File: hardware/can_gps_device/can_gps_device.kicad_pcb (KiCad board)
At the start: 2 copper layers, 70 x 55 mm, 79 parts, among them J1 AMP_Superseal_9-6437287-8, J2 TC2030, U1 STM32F042K6Ux, U2 TLE42744DV33ATMA1, U3 TCAN3403DRQ1, U4 R-78E5.0-0.5, Y1 ECS-160-10-36Q-AES-TR

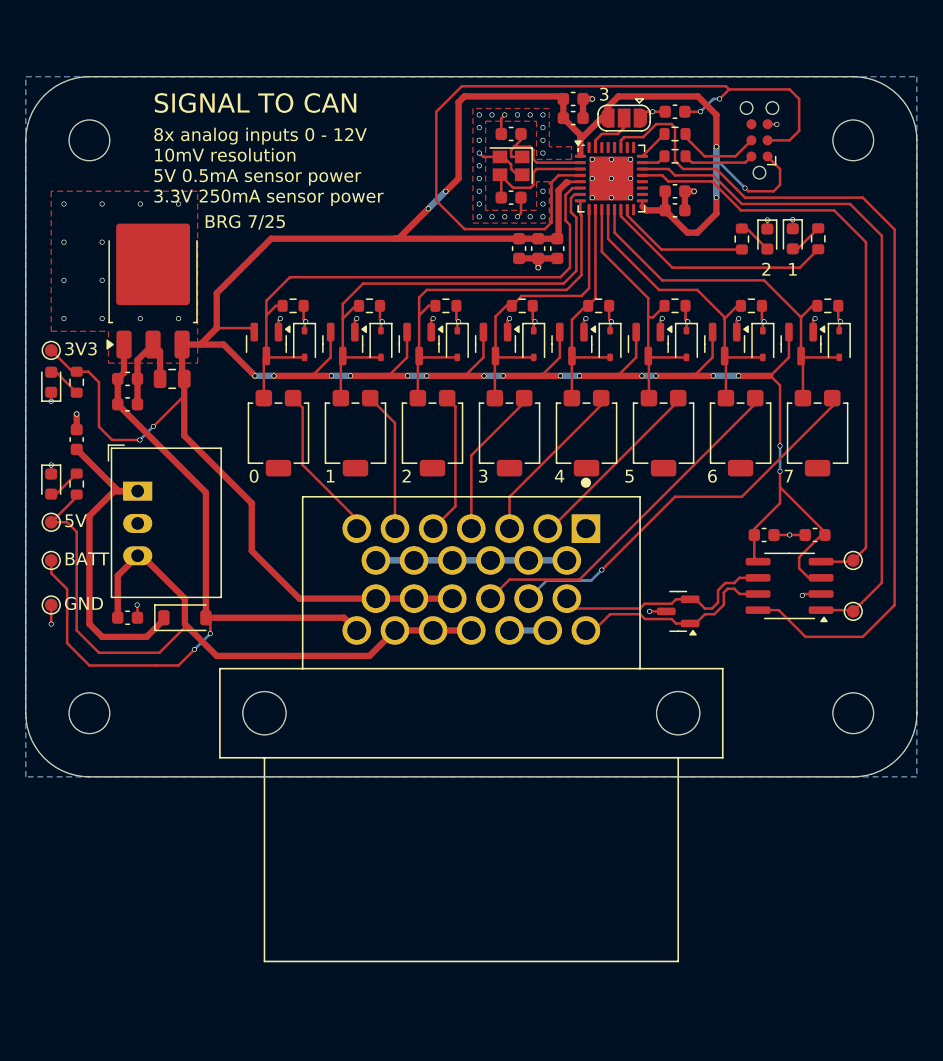
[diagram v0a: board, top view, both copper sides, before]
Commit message: Schematic Initial Rev
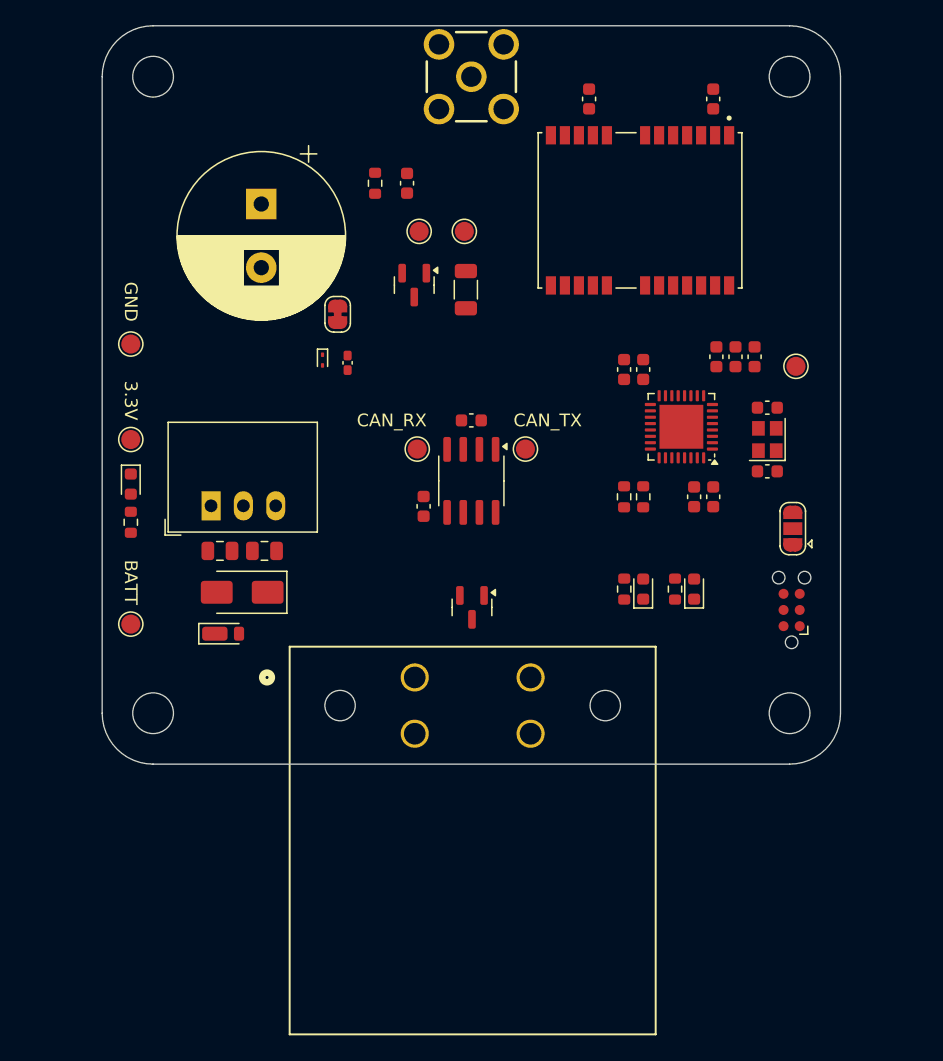
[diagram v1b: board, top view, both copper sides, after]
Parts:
- removed D10, D11, D12, D17, D18, D19, D20, D9: BAT54S, Package_TO_SOT_SMD:SOT-23
- removed D13, D14, D15, D16: PESD3V3L1BA, Diode_SMD:D_SOD-323
- removed D21: CDBW140-G, Diode_SMD:D_SOD-123
- removed D22: LED, LED_SMD:LED_0603_1608Metric
- removed R10, R11, R12, R13, R8, R9: 6.8k, Resistor_SMD:R_0603_1608Metric
- removed R14: 1k, Resistor_SMD:R_0603_1608Metric
- removed RV1, RV2, RV3, RV4, RV5, RV6, RV7, RV8: 3314G-1-503E, Potentiometer_SMD:Potentiometer_Bourns_3314G_Vertical
- removed TP3: 3.3V, TestPoint:TestPoint_Pad_D1.0mm
- removed TP4: CAN_TX, TestPoint:TestPoint_Pad_D1.0mm
- removed TP5: CAN_RX, TestPoint:TestPoint_Pad_D1.0mm
- removed TP6: TestPoint, TestPoint:TestPoint_Pad_D1.0mm
- added 3.3V1: TestPoint, TestPoint:TestPoint_Pad_D1.5mm, F.Cu at (123.2, 103.5)
- added BATT1: TestPoint, TestPoint:TestPoint_Pad_D1.5mm, F.Cu at (123.2, 118.0)
- added GND1: TestPoint, TestPoint:TestPoint_Pad_D1.5mm, F.Cu at (123.2, 96.0)
- added J3: SMA-J-P-X-RA-TH1, can_gps_device:SAMTEC_SMA-J-P-X-RA-TH1, F.Cu at (150.0, 75.0)
- added JP2: Jumper_2_Bridged, Jumper:SolderJumper-2_P1.3mm_Bridged_RoundedPad1.0x1.5mm, F.Cu at (139.5, 93.7)
- added L1: LQG15HN27NJ02D, Inductor_SMD:L_0402_1005Metric_Pad0.77x0.64mm_HandSolder, F.Cu at (140.3, 97.5)
- added MCU_RX1: TestPoint, TestPoint:TestPoint_Pad_D1.5mm, F.Cu at (149.4, 87.2)
- added MCU_TX1: TestPoint, TestPoint:TestPoint_Pad_D1.5mm, F.Cu at (145.9, 87.2)
- added RESET1: TestPoint, TestPoint:TestPoint_Pad_D1.5mm, F.Cu at (175.5, 97.8)
- C10, C11: value 1uF -> 0.1uF
- C12: value 0.1uF -> 1uF
- C13: value 22uF -> 0.1uF; footprint Capacitor_SMD:C_0805_2012Metric -> Capacitor_SMD:C_0603_1608Metric
- C14: value 0.1uF -> 100nF 16V X7R
- C15: value 0.1uF -> FYD0H104ZF; footprint Capacitor_SMD:C_0603_1608Metric -> Capacitor_THT:CP_Radial_D13.0mm_P5.00mm
- C16, C17: footprint Capacitor_SMD:C_0603_1608Metric -> Capacitor_SMD:C_0805_2012Metric
- C2: value 4.7uF -> 0.1uF
- C4: value 0.1uF -> 4.7uF
- C6: value 0.1uF -> 12pF
- C7: value 12pF -> 10nF
- C8: value 10nF -> 12pF
- C9: value 12pF -> 1uF
- D1, D2: value LED -> Green LED
- D3: value LED -> NUP2105L; footprint LED_SMD:LED_0603_1608Metric -> Package_TO_SOT_SMD:SOT-23
- D4: value NUP2105L -> BAT54A
- D5: value PESD3V3L1BA -> ESD9R3.3ST5G; footprint Diode_SMD:D_SOD-323 -> Diode_SMD:D_SOD-923
- D6: value PESD3V3L1BA -> RSX051VYM30FHTR; footprint Diode_SMD:D_SOD-323 -> Diode_SMD:D_TUMD2
- D7: value PESD3V3L1BA -> P4SMAJ28CA-AQ; footprint Diode_SMD:D_SOD-323 -> Diode_SMD:D_SMA
- D8: value PESD3V3L1BA -> Green LED; footprint Diode_SMD:D_SOD-323 -> LED_SMD:LED_0603_1608Metric
- J1: value AMP_Superseal_9-6437287-8 -> Conn_01x04; footprint signal_to_can:TE_9-6437287-8_1 -> can_gps_device:ATF13-4P-BM13_AMP
- R5: value 1k -> 22 1/2 W 1206; footprint Resistor_SMD:R_0603_1608Metric -> Resistor_SMD:R_1206_3216Metric
- R6: value 6.8k -> 470
- R7: value 6.8k -> 1k
- TP1: value POWER_INPUT -> CAN_TX; footprint TestPoint:TestPoint_Pad_D1.0mm -> TestPoint:TestPoint_Pad_D1.5mm
- TP2: value GND -> CAN_RX; footprint TestPoint:TestPoint_Pad_D1.0mm -> TestPoint:TestPoint_Pad_D1.5mm
- U2: value TLE42744DV33ATMA1 -> TCAN3403DRQ1; footprint Package_TO_SOT_SMD:TO-252-3_TabPin2 -> Package_SO:SOIC-8_3.9x4.9mm_P1.27mm
- U3: value TCAN3403DRQ1 -> NEO-M9V-20B; footprint Package_SO:SOIC-8_3.9x4.9mm_P1.27mm -> can_gps_device:XCVR_NEO-M9V-20B
- U4: value R-78E5.0-0.5 -> R-78E3.3-0.5
- moved H2 74.3 mm to (175.0, 75.0)
- moved H3 71.1 mm to (125.0, 125.0)
- moved C12 51.9 mm to (169.0, 76.8), turned to 90 degrees
- moved C15 47.3 mm to (133.5, 85.0), turned to -90 degrees
- moved C14 42.3 mm to (144.9, 83.4), turned to -90 degrees
- moved C13 39.4 mm to (159.2, 76.8), turned to 90 degrees
- moved TP1 38.3 mm to (154.2, 104.2)
- moved D3 37.5 mm to (150.1, 116.7), turned to -90 degrees
- moved J2 37.0 mm to (175.2, 116.9)
- moved JP1 34.9 mm to (175.2, 110.5), turned to 90 degrees
- moved D8 33.5 mm to (123.2, 107.0)
- moved D4 33.0 mm to (145.5, 91.4), turned to -90 degrees
- moved U3 31.8 mm to (163.2, 85.5), turned to -90 degrees
- moved R5 31.4 mm to (149.6, 91.7)
- moved TP2 31.3 mm to (145.8, 104.2)
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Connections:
- C1 pad 1: +3V3 -> +3.3V
- C11 pad 1: GND -> +3V3
- C11 pad 2: +BATT -> GND
- C12 pad 1: GND -> +3V3
- C12 pad 2: +BATT -> GND
- C13 pad 1: +3V3 -> +BATT_BCKP
- C14 pad 1: +3V3 -> Net-(C14-Pad1)
- C15 pad 1: +3V3 -> +BATT_BCKP
- C16 pad 1: Net-(D21-K) -> Net-(D6-K)
- C17 pad 1: +5V -> +3V3
- C2 pad 1: +3V3 -> /Microcontroller/NRST
- C3 pad 1: /Microcontroller/NRST -> +3.3V
- C4 pad 1: +3V3 -> +3.3V
- C5 pad 1: +3V3 -> +3.3V
- C6 pad 1: +3V3 -> GND
- C6 pad 2: GND -> /Microcontroller/OSC_IN
- C7 pad 1: GND -> +3.3V
- C7 pad 2: /Microcontroller/OSC_IN -> GND
- C8 pad 1: +3V3 -> /Microcontroller/OSC_OUT
- C9 pad 1: /Microcontroller/OSC_OUT -> +3.3V
- D3 pad 1: GND -> /CAN_P
- D3 pad 2: Net-(D3-A) -> /CAN_N
- D4 pad 1: /CAN_P -> unconnected-(D4-Pad1)
- D4 pad 2: /CAN_N -> Net-(D4-Pad2)
- D4 pad 3: GND -> +3.3V
- D5 pad 2: /3.3V_ANALOG_INPUT_0 -> /GPS Module/RF_IN
- D6 pad 1: GND -> Net-(D6-K)
- D6 pad 2: /3.3V_ANALOG_INPUT_1 -> +BATT
- D7 pad 2: /3.3V_ANALOG_INPUT_2 -> Net-(D6-K)
- D8 pad 2: /3.3V_ANALOG_INPUT_3 -> Net-(D8-A)
- J1 pad 1: GND -> +BATT
- J1 pad 2: /12V_ANALOG_INPUT_5 -> /CAN_P
- J1 pad 3: /12V_ANALOG_INPUT_4 -> /CAN_N
- J1 pad 4: /12V_ANALOG_INPUT_3 -> GND
- J2 pad 1: +3V3 -> +3.3V
- JP1 pad 3: +3V3 -> +3.3V
- R5 pad 1: +3V3 -> Net-(C14-Pad1)
- R5 pad 2: Net-(D3-A) -> /GPS Module/VCC_RF
- R6 pad 1: /3.3V_ANALOG_INPUT_0 -> Net-(D4-Pad2)
- R6 pad 2: GND -> +BATT_BCKP
- R7 pad 1: /3.3V_ANALOG_INPUT_1 -> +3V3
- R7 pad 2: GND -> Net-(D8-A)
- TP1 pad 1: +BATT -> /CAN_TX
- TP2 pad 1: GND -> /CAN_RX
- U1 pad 1: +3V3 -> +3.3V
- U1 pad 10: /3.3V_ANALOG_INPUT_4 -> unconnected-(U1-PA4-Pad10)
- U1 pad 11: /3.3V_ANALOG_INPUT_5 -> unconnected-(U1-PA5-Pad11)
- U1 pad 12: /3.3V_ANALOG_INPUT_6 -> unconnected-(U1-PA6-Pad12)
- U1 pad 13: /3.3V_ANALOG_INPUT_7 -> unconnected-(U1-PA7-Pad13)
- U1 pad 14: /Microcontroller/LED_STATUS_1 -> /GNSS_TIMEPULSE
- U1 pad 15: /Microcontroller/LED_STATUS_2 -> /GNSS_RESET
- U1 pad 16: unconnected-(U1-PB2-Pad16) -> /GNSS_WAKE_ON_MOTION
- U1 pad 17: +3V3 -> +3.3V
- U1 pad 19: unconnected-(U1-PA9-Pad19) -> /UART_MCU_TX
- U1 pad 20: unconnected-(U1-PA10-Pad20) -> /UART_MCU_RX
- U1 pad 25: unconnected-(U1-PA15-Pad25) -> /CAN_STANDBY
- U1 pad 26: unconnected-(U1-PB3-Pad26) -> /Microcontroller/LED_STATUS_2
- U1 pad 27: /CAN_STANDBY -> /Microcontroller/LED_STATUS_1
- U1 pad 5: +3V3 -> +3.3V
- U1 pad 6: /3.3V_ANALOG_INPUT_0 -> unconnected-(U1-PA0-Pad6)
- U1 pad 7: /3.3V_ANALOG_INPUT_1 -> unconnected-(U1-PA1-Pad7)
- U1 pad 8: /3.3V_ANALOG_INPUT_2 -> unconnected-(U1-PA2-Pad8)
- U1 pad 9: /3.3V_ANALOG_INPUT_3 -> unconnected-(U1-PA3-Pad9)
- U2 pad 1: +BATT -> /CAN_TX
- U3 pad 1: /CAN_TX -> unconnected-(U3-~{SAFEBOOT}-Pad1)
- U3 pad 2: GND -> +3V3
- U3 pad 3: +3V3 -> /GNSS_TIMEPULSE
- U3 pad 4: /CAN_RX -> unconnected-(U3-WHEELTICK-Pad4)
- U3 pad 5: +3V3 -> unconnected-(U3-USB_DM-Pad5)
- U3 pad 6: /CAN_N -> unconnected-(U3-USB_DP-Pad6)
- U3 pad 7: /CAN_P -> GND
- U3 pad 8: /CAN_STANDBY -> /GNSS_RESET
- U4 pad 1: Net-(D21-K) -> Net-(D6-K)
- U4 pad 3: +5V -> +3V3
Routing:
- net +3V3: track 263.7 -> 0.00 mm, vias 23 -> 0
- net GND: track 82.1 -> 0.00 mm, vias 76 -> 0
- net /CAN_STANDBY: track 69.7 -> 0.00 mm
- net /Microcontroller/NRST: track 62.1 -> 0.00 mm, vias 2 -> 0
- net +5V: track 60.4 -> 0.00 mm
- net +BATT: track 58.2 -> 0.00 mm, vias 2 -> 0
- net /CAN_TX: track 54.0 -> 0.00 mm
- net /CAN_RX: track 47.7 -> 0.00 mm
- net /3.3V_ANALOG_INPUT_0: track 44.5 -> 0.00 mm
- net /3.3V_ANALOG_INPUT_1: track 38.4 -> 0.00 mm
- net /3.3V_ANALOG_INPUT_2: track 31.9 -> 0.00 mm
- net /12V_ANALOG_INPUT_7: track 30.8 -> 0.00 mm, vias 1 -> 0
- net /3.3V_ANALOG_INPUT_7: track 30.3 -> 0.00 mm
- net /12V_ANALOG_INPUT_6: track 27.6 -> 0.00 mm
- net Net-(D21-K): track 26.2 -> 0.00 mm
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- removed copper zone on B.Cu, net GND
- removed copper zone on F.Cu, net GND
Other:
- board size 70 x 55 mm -> 58 x 58 mm
- board text added: "3.3V"
- board text added: "CAN_RX"
- board text added: "CAN_TX"
- board text removed: "0"
- board text removed: "1"
- board text removed: "2"
- board text removed: "3"
- board text removed: "3V3"
- board text removed: "4"
- board text removed: "5"
- board text removed: "5V"
- board text removed: "6"
- board text removed: "7"
- board text removed: "8x analog inputs 0 - 12V 10mV resolution 5V 0.5mA sensor power 3.3V 250mA sensor power"
- board text removed: "BRG 7/25"
- board text removed: "SIGNAL TO CAN"
